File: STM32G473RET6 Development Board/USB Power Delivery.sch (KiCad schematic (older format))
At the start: 19 parts, among them J1 Screw_Terminal_01x02, J2 USB_C_Receptacle_USB2.0, Q1 DMP3013SFV, Q2 IRF9394M, Q3 IRF9394M, SW2 SW_DIP_x02, U2 INA260

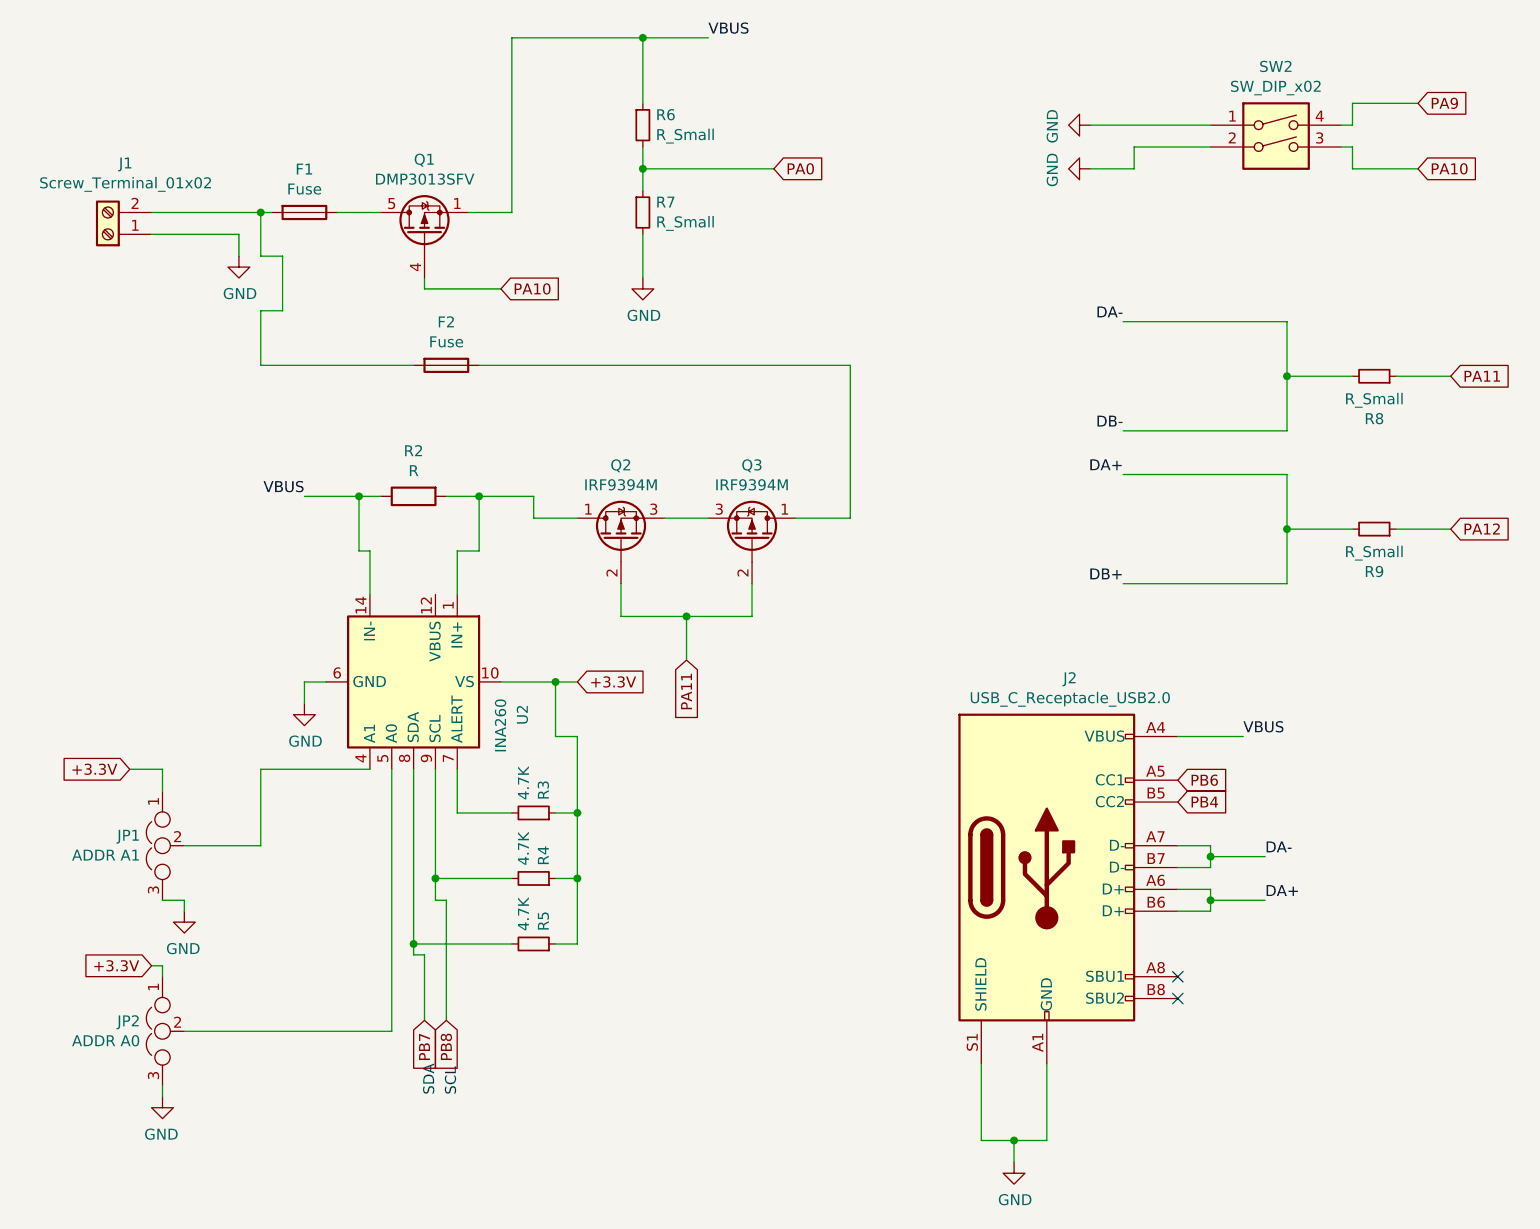
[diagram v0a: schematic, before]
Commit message: Add files via upload
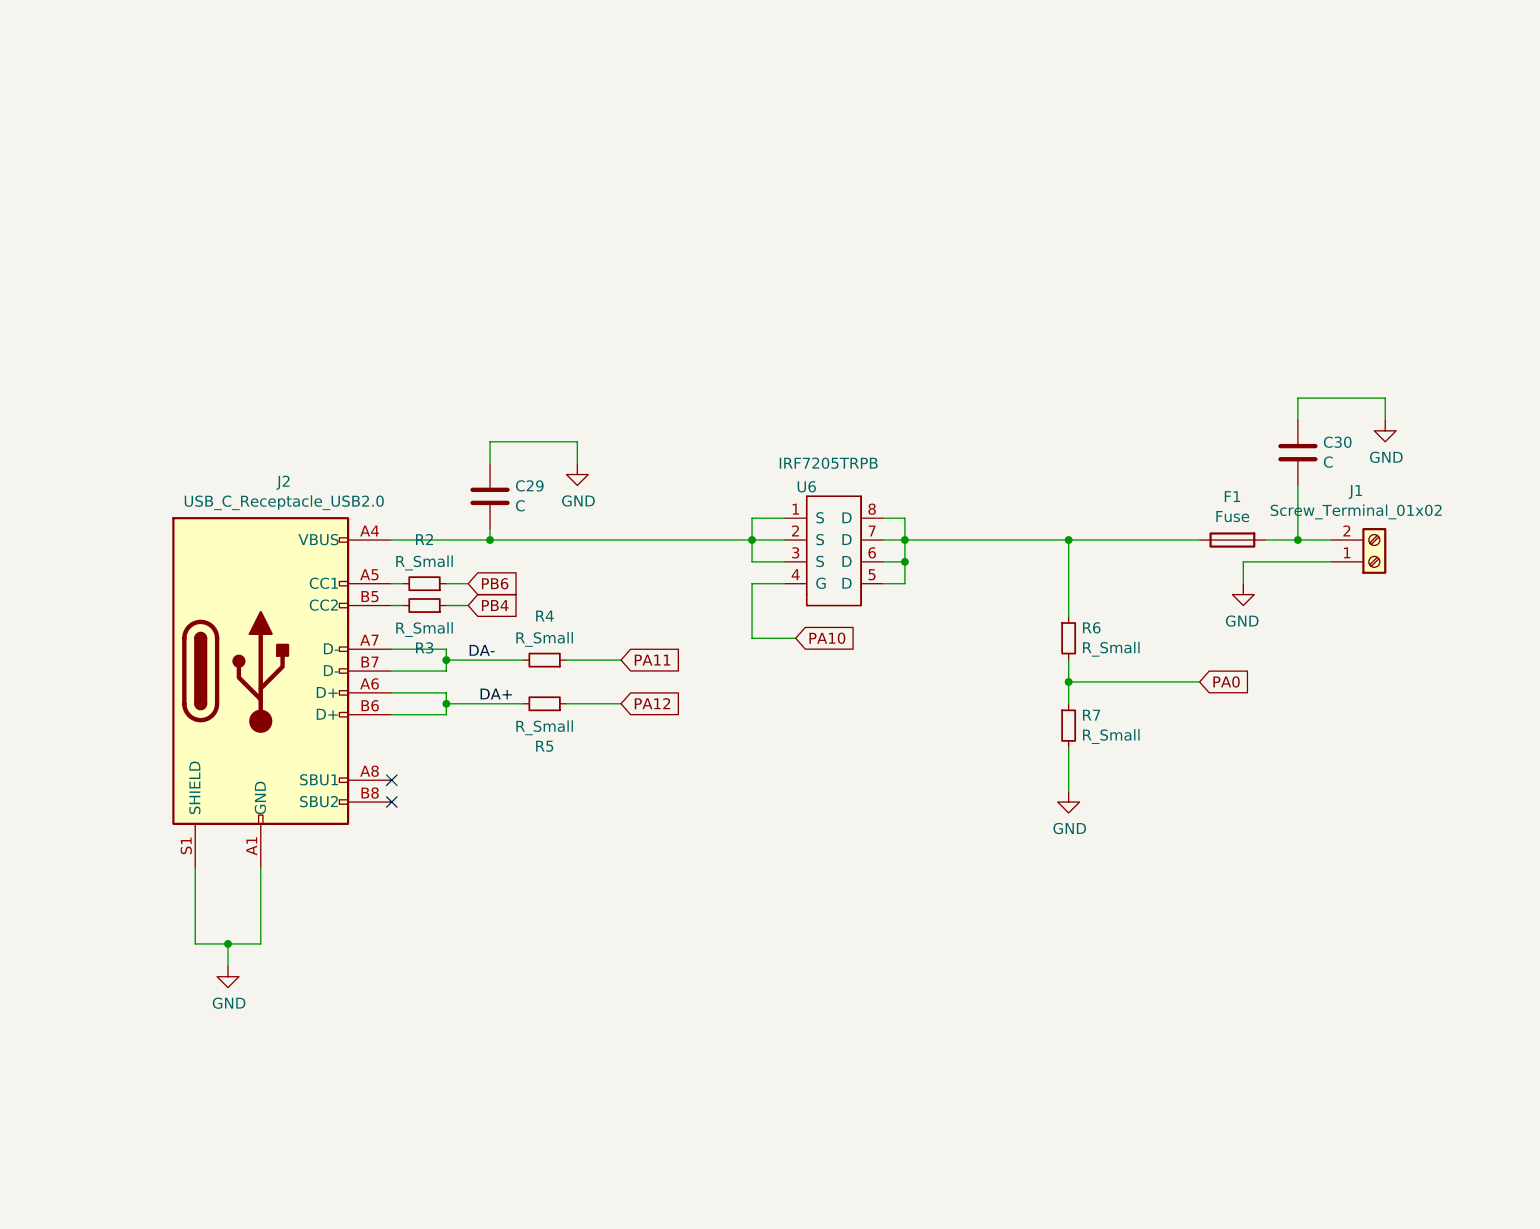
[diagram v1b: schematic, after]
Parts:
- removed F2: Fuse, Fuse:Fuse_0603_1608Metric, symbol Device:Fuse
- removed JP1: ADDR A1, Button_Switch_SMD:SW_DIP_SPSTx02_Slide_Copal_CHS-02A_W5.08mm_P1.27mm_JPin, symbol Device:Jumper_NC_Dual
- removed JP2: ADDR A0, Button_Switch_SMD:SW_DIP_SPSTx02_Slide_Copal_CHS-02A_W5.08mm_P1.27mm_JPin, symbol Device:Jumper_NC_Dual
- removed Q1: DMP3013SFV, Package_SON:Diodes_PowerDI3333-8, symbol Transistor_FET:DMP3013SFV
- removed Q2, Q3: IRF9394M, Package_DirectFET:DirectFET_MC, symbol Transistor_FET:IRF9394M
- removed R2: R, Resistor_SMD:R_0603_1608Metric, symbol Device:R
- removed R8, R9: R_Small, Resistor_SMD:R_0603_1608Metric, symbol Device:R_Small
- removed SW2: SW_DIP_x02, Button_Switch_SMD:SW_DIP_SPSTx02_Slide_6.7x6.64mm_W8.61mm_P2.54mm_LowProfile, symbol Switch:SW_DIP_x02
- removed U2: INA260, Package_SO:TSSOP-16_4.4x5mm_P0.65mm, symbol Sensor:INA260
- added C29, C30: C, Capacitor_SMD:CP_Elec_3x5.3, symbol Device:C
- added R2: R_Small, Resistor_SMD:R_0603_1608Metric, symbol Device:R_Small
- added U6: IRF7205TRPB, Package_SO:SOP-8_3.9x4.9mm_P1.27mm, symbol Transistor_FET:IRF7205TRPB
- R3, R4, R5: value 4.7K -> R_Small
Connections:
- net PB7 is gone; now on net DA+: R5.2
- net PB8 is gone; now on net DA-: R4.2
- net GND: now also C29.1, C30.1
- net PA10: now also U6.4 (G)
- net PA11: now also R4.1
- net PA12: now also R5.1
- net PB4: now also R3.1; no longer J2.B5 (CC2)
- net PB6: now also R2.1; no longer J2.A5 (CC1)
- net at F1.2, J1.2 (Pin_2): now also C30.2
- net at F1.1: now also R6.1, U6.5 (D), U6.6 (D), U6.7 (D), U6.8 (D)
- net at R3.2: now also J2.B5 (CC2)
- removed net +3.3V: R3.1, R4.1, R5.1
- net VBUS: no longer names the net of J2.A4 (VBUS), J2.A9 (VBUS), J2.B4 (VBUS), J2.B9 (VBUS)
- net VBUS: now also C29.2, U6.1 (S), U6.2 (S), U6.3 (S); no longer R6.1
- new net: J2.A5 (CC1), R2.2
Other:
- note removed: "SCL\n"
- note removed: "SDA"
- moved on the sheet: F1, J1, R6, R7
